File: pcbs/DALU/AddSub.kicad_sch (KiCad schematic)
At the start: 14 parts, among them U401 74HC86, U402 74HC08, U403 74HC86, U404 74HC86, U405 74HC283, U406 74HC283, U407 74HC245, U408 74HC245

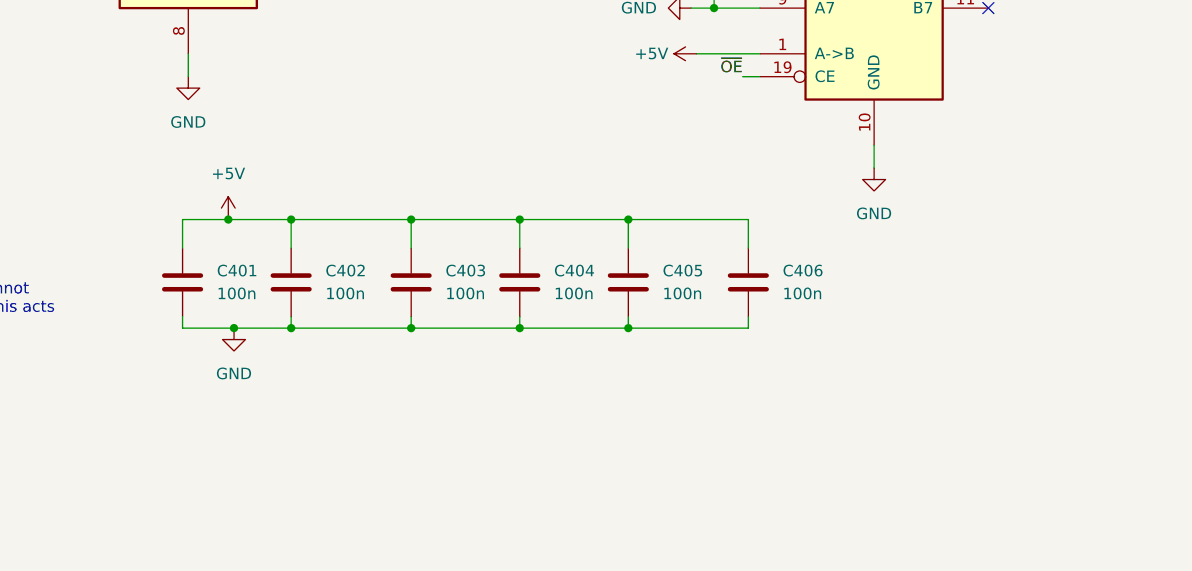
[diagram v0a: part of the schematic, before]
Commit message: Finish preliminary routing
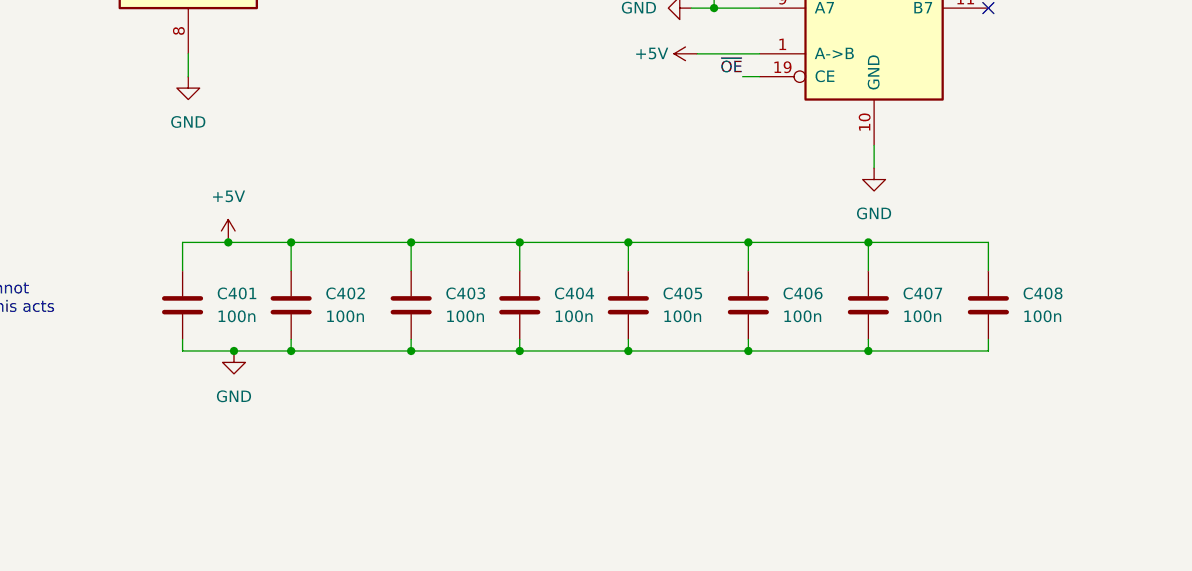
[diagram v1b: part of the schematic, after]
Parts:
- added C407, C408: 100n, Capacitor_SMD:C_0603_1608Metric, symbol Device:C
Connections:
- net +5V: now also C407.1, C408.1
- net GND: now also C407.2, C408.2
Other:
- moved on the sheet: C401, C402, C403, C404, C405, C406
